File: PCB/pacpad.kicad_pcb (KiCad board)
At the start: 2 copper layers, 68 x 65 mm, 9 parts, among them SW1 SW_Push, SW2 SW_Push, SW3 SW_Push, SW4 SW_Push, SW5 RotaryEncoder_Switch, U1 MOUDLE-SEEEDUINO-XIAO, U2 ER_OLEDM0.91_1x-I2C

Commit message: Added gerbers in production
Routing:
- net Net-(D1-DIN): vias 3 -> 2
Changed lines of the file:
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@@
-		(net "Net-(D1-DIN)")
-	)
-	(via
-		(at 161.5 50)
-		(size 0.6)
-		(drill 0.3)
-		(layers "F.Cu" "B.Cu")
 		(net "Net-(D1-DIN)")
 	)

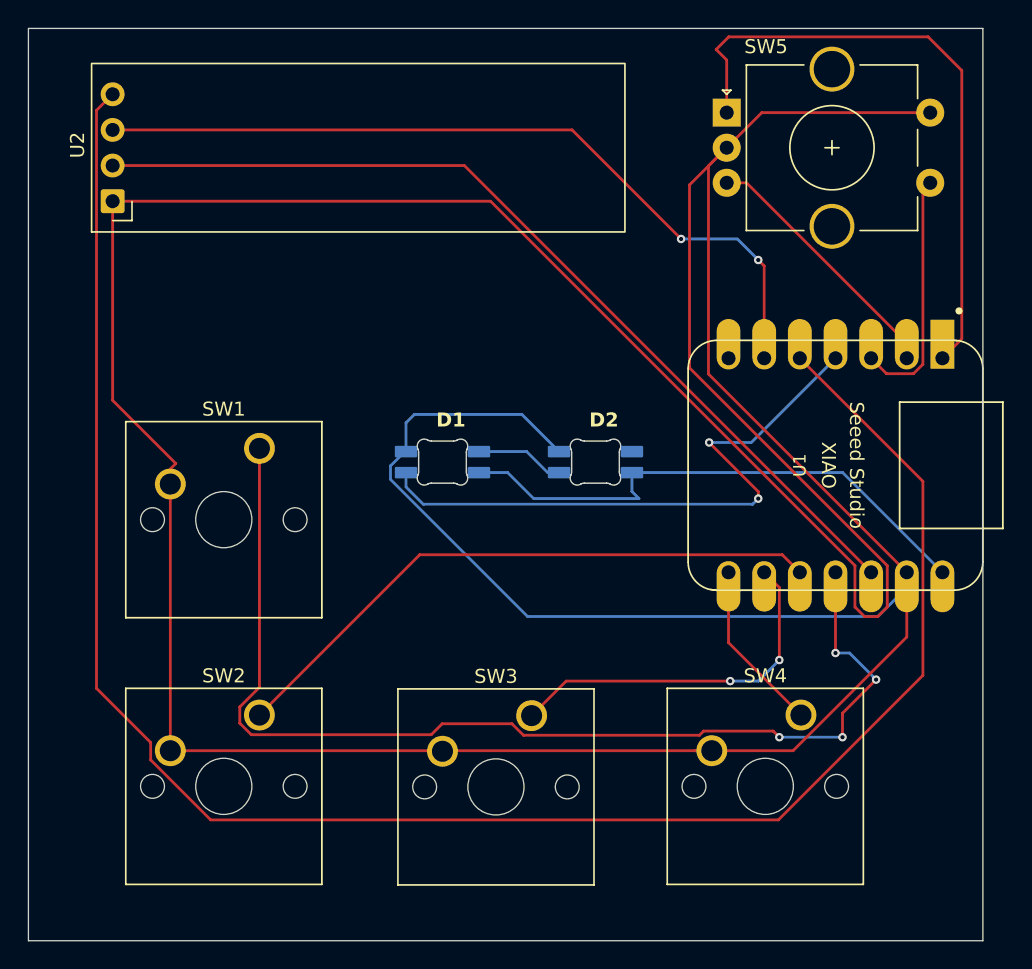
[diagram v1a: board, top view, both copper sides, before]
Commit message: Update: PCB with gerbers.zip
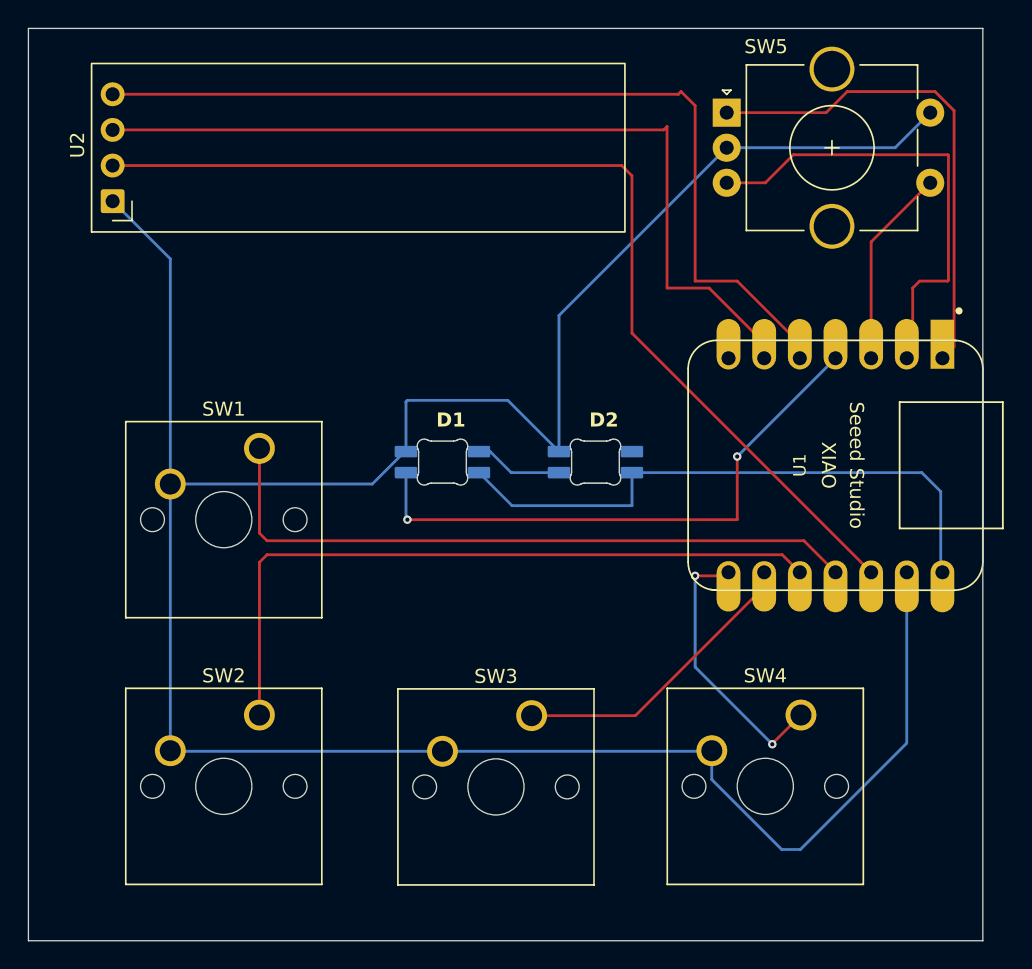
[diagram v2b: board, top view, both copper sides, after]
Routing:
- net GND: track 324.2 -> 188.7 mm
- net Net-(U1-PA8_A4_D4_SDA): track 136.8 -> 64.8 mm
- net Net-(U1-PA6_A10_D10_MOSI): track 78.9 -> 48.2 mm, vias 4 -> 0
- net Net-(U1-PA4_A1_D1): track 18.6 -> 33.5 mm
- net Net-(U1-PA02_A0_D0): track 44.7 -> 35.4 mm
- net Net-(U1-PB09_A7_D7_RX): track 12.3 -> 19.7 mm, vias 0 -> 2
- net Net-(U1-3V3): track 66.0 -> 72.6 mm
- net Net-(U1-PA5_A9_D9_MISO): track 43.7 -> 50.1 mm
- net Net-(U1-PA7_A8_D8_SCK): track 27.0 -> 21.4 mm, vias 2 -> 0
- net Net-(D1-DIN): track 46.2 -> 41.3 mm
- net Net-(U1-PA9_A5_D5_SCL): track 57.0 -> 60.7 mm, vias 2 -> 0
- net Net-(U1-PA10_A2_D2): track 17.6 -> 14.2 mm
- net Net-(D1-VDD): track 41.3 -> 42.6 mm
